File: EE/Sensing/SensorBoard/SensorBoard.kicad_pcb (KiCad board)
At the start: 2 copper layers, 113 parts, among them J1 Conn_02x13_Odd_Even, J101 Peg, J102 Peg, J11 Peg, J12 Peg, J21 Peg, J22 Peg, J31 Peg, J32 Peg, J41 Peg, J42 Peg, J51 Peg, J52 Peg, J61 Peg, J62 Peg, J71 Peg, J72 Peg, J81 Peg, J82 Peg, J91 Peg, J92 Peg, Q1 BSS84DW, Q10 BSS84DW, Q2 BSS84DW, Q3 BSS84DW, Q4 BSS84DW, Q5 BSS84DW, Q6 BSS84DW, Q7 BSS84DW, Q8 BSS84DW, Q9 BSS84DW, U1 TCR2EE27, U101 AH1381, U102 AH1381, U11 AH1381, U12 AH1381, U2 TCR2EE32, U21 AH1381, U22 AH1381, U31 AH1381, U32 AH1381, U41 AH1381, U42 AH1381, U51 AH1381, U52 AH1381, U61 AH1381, U62 AH1381, U71 AH1381, U72 AH1381, U81 AH1381, U82 AH1381, U91 AH1381, U92 AH1381

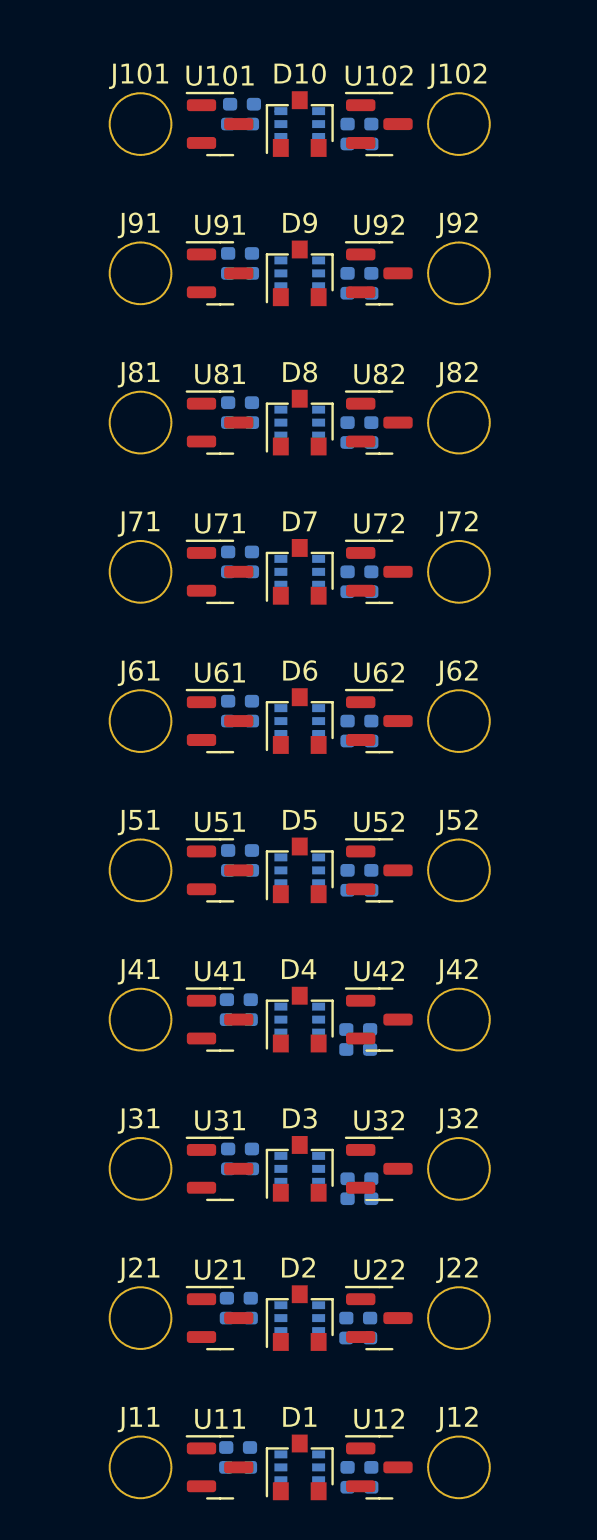
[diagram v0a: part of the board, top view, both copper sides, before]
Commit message: More Layout
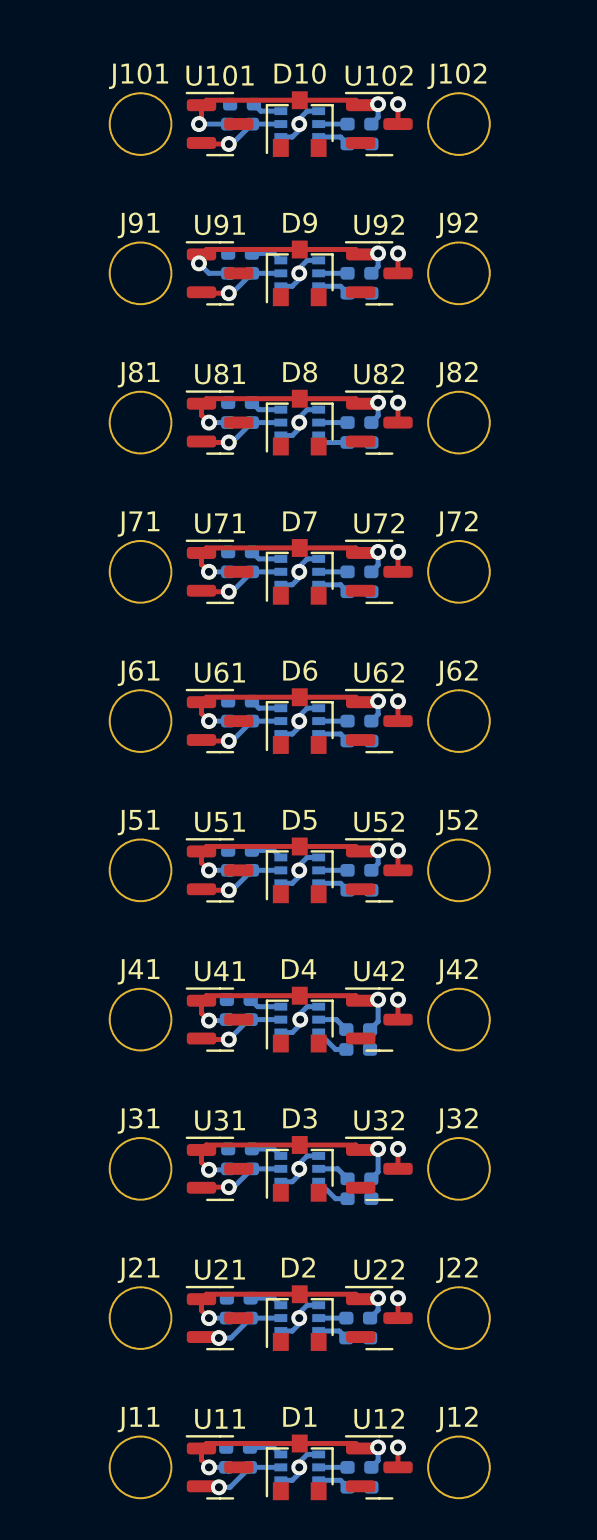
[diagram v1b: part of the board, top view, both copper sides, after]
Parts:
- turned R31 to 0 degrees
- turned R32 to 180 degrees
- turned R36 to 180 degrees
- turned R5 to 0 degrees
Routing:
- net /2v7: track 2.91 -> 127.5 mm, vias 0 -> 20
- net GND: track 8.34 -> 45.9 mm, vias 8 -> 28
- net /B1_0_4: track 0.00 -> 4.42 mm, vias 0 -> 1
- net /B1_0_3: track 0.00 -> 4.42 mm, vias 0 -> 1
- net /B1_0_2: track 0.00 -> 4.42 mm, vias 0 -> 1
- net /B1_0_1: track 0.00 -> 4.42 mm, vias 0 -> 1
- net /B1_0_0: track 0.00 -> 4.42 mm, vias 0 -> 1
- net /B0_0_4: track 0.00 -> 4.42 mm, vias 0 -> 1
- net /B0_0_3: track 0.00 -> 4.42 mm, vias 0 -> 1
- net /B0_0_1: track 0.00 -> 4.42 mm, vias 0 -> 1
- net /B0_0_0: track 0.00 -> 4.42 mm, vias 0 -> 1
- net /B0_0_2: track 0.00 -> 4.38 mm, vias 0 -> 1
- net Net-(Q3-Pad6): track 0.00 -> 1.80 mm
- net Net-(Q4-Pad6): track 0.00 -> 1.74 mm
- net Net-(Q1-Pad3): track 0.00 -> 1.69 mm
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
